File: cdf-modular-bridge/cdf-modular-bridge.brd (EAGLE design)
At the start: 50.8 x 38.1 mm, 16 parts

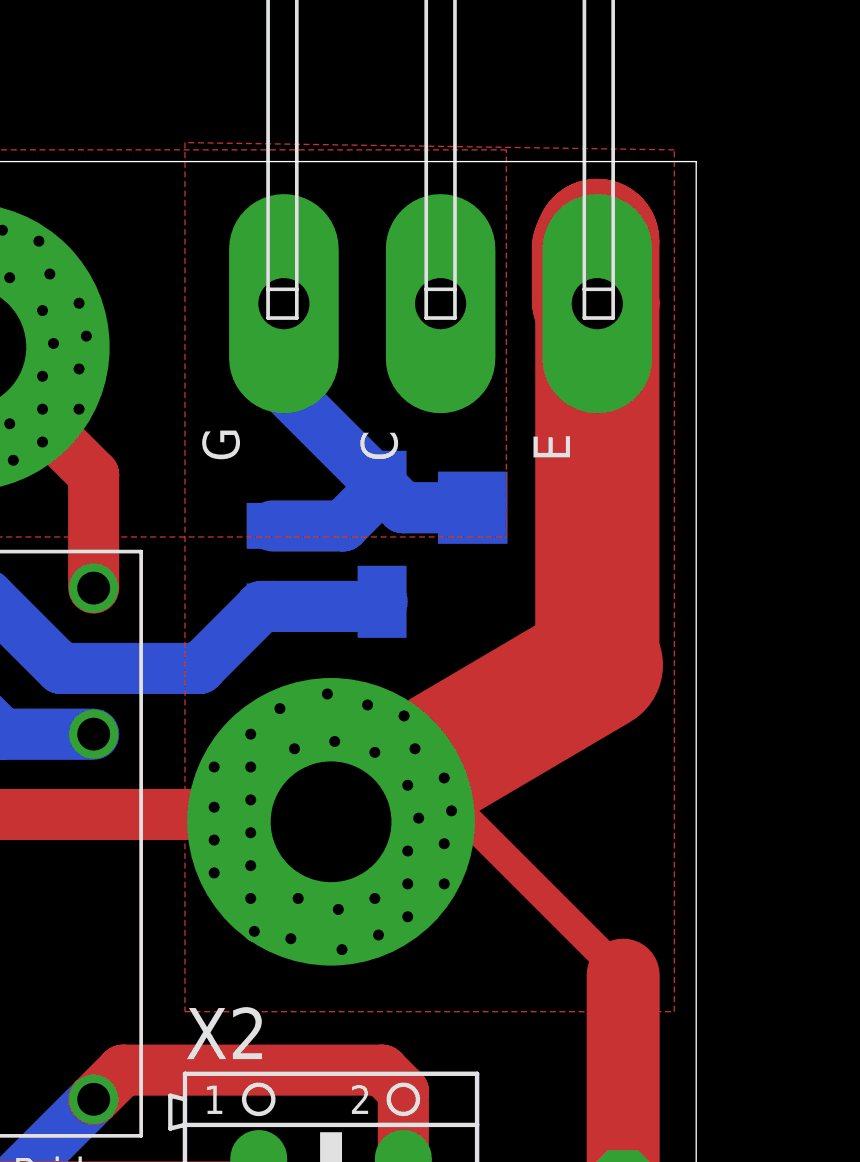
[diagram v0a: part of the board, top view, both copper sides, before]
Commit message: wip
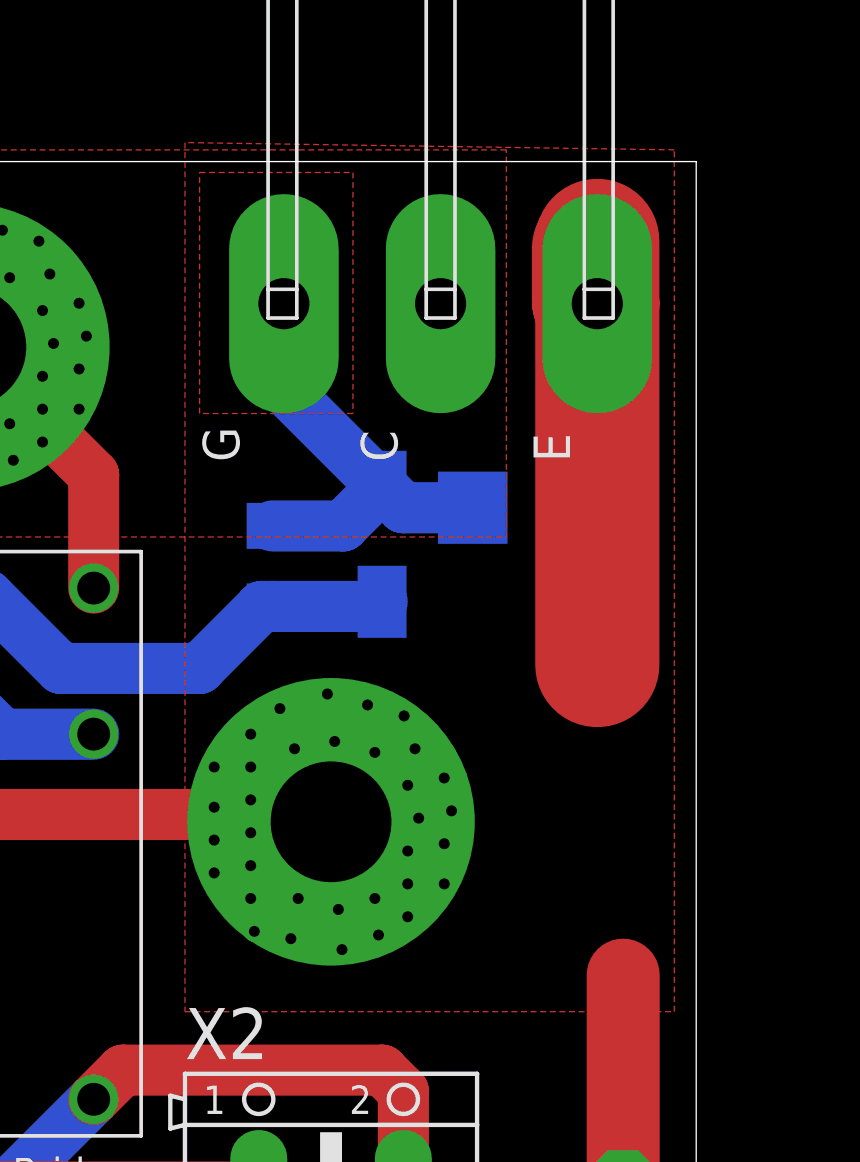
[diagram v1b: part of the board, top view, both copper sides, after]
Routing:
- net DC-: track 69.6 -> 50.3 mm
- added copper zone on layer 1, net N$5
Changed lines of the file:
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@@
 </class>
 </classes>
-<designrules name="oshpark">
+<designrules name="oshpark *">
 <description language="de">&lt;b&gt;EAGLE Design Rules&lt;/b&gt;
 &lt;p&gt;
@@
 <param name="dpGapFactor" value="2.5"/>
 <param name="checkGrid" value="0"/>
-<param name="checkAngle" value="0"/>
+<param name="checkAngle" value="1"/>
 <param name="checkFont" value="1"/>
 <param name="checkRestrict" value="1"/>
@@
 <contactref element="U$2" pad="C"/>
 <contactref element="OUT" pad="X"/>
-<polygon width="0.254" layer="1" isolate="0.381" thermals="no">
+<polygon width="0.254" layer="1" isolate="0.381" thermals="no" rank="2">
 <vertex x="44.196" y="38.5064"/>
 <vertex x="12.446" y="38.5064"/>
@@
 <wire x1="36.46" y1="33.1584" x2="36.46" y2="30.2084" width="1.778" layer="16"/>
 <wire x1="36.46" y1="30.2084" x2="39.878" y2="26.7904" width="1.778" layer="16"/>
+<polygon width="0.254" layer="1">
+<vertex x="33.528" y="37.719"/>
+<vertex x="38.862" y="37.719"/>
+<vertex x="38.862" y="29.337"/>
+<vertex x="33.528" y="29.337"/>
+</polygon>
 </signal>
 <signal name="DC-">
@@
 <contactref element="U$2" pad="E"/>
 <contactref element="DC-" pad="X"/>
-<wire x1="47.36" y1="20.5884" x2="38.854609375" y2="15.582528125" width="4.572" layer="1"/>
-<wire x1="38.854609375" y1="15.582528125" x2="38.1" y2="15.1384" width="4.572" layer="1"/>
 <wire x1="47.36" y1="20.5884" x2="47.36" y2="33.1584" width="4.318" layer="1"/>
 <wire x1="47.36" y1="33.1584" x2="47.36" y2="35.3424" width="4.318" layer="1"/>
-<wire x1="47.36" y1="35.3424" x2="47.244" y2="35.0774" width="4.318" layer="1"/>
 <wire x1="47.244" y1="35.0774" x2="47.244" y2="33.2744" width="4.318" layer="1"/>
 <wire x1="47.244" y1="33.2744" x2="47.36" y2="33.1584" width="4.318" layer="1"/>
-<polygon width="0.254" layer="1" isolate="0.381" thermals="no" rank="2">
+<polygon width="0.254" layer="1" isolate="0.381" thermals="no" rank="3">
 <vertex x="50.038" y="38.5064"/>
 <vertex x="33.02" y="38.7604"/>
@@
 <wire x1="37.846" y1="15.3924" x2="38.1" y2="15.1384" width="1.778" layer="1"/>
 <contactref element="TP2" pad="TP"/>
-<wire x1="48.26" y1="9.8044" x2="42.418" y2="15.6464" width="1.016" layer="1"/>
 <wire x1="48.26" y1="2.4384" x2="48.26" y2="9.8044" width="2.54" layer="1"/>
 <contactref element="DC-" pad="X@1"/>
@@
 <wire x1="8.89" y1="18.9484" x2="8.89" y2="33.1584" width="4.318" layer="1"/>
 <wire x1="8.89" y1="35.4584" x2="8.89" y2="33.1584" width="4.318" layer="1"/>
-<polygon width="0.254" layer="1" isolate="0.381" thermals="no" rank="2">
+<polygon width="0.254" layer="1" isolate="0.381" thermals="no" rank="3">
 <vertex x="18.288" y="38.2524"/>
 <vertex x="5.588" y="38.2524"/>
